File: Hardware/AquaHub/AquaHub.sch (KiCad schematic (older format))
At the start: 73 parts, among them J10 PinHeader6, J13 PinHeader2, J14 PinHeader3, Q2 2SC1815, SW1 SW_Push, SW2 SW_Push, SW3 SW_Push, SW4 SW_Push, SW5 SW_Push, SW6 SW_Push, U1 ESP32-WROOM, U3 1A 3.3V, U4 Low-Side Driver, U5 1A 5V, U6 TCA9534, U7 DS1307+, U8 TPIC2810D, Y1 32.768KHz

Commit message: Commit latest hardware updates and initial firmware
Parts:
- BT1: footprint AquaFootprints:Multicomp-BC-2001 -> Battery:BatteryHolder_Multicomp_BC-2001_1x2032; Mouser (none) -> 534-1058; manf# (none) -> x
- C3: Mouser (none) -> TAJB106K006SNJ; manf# TAJB106K006SNJ -> (none)
- C4: Farnell (none) -> CA06848; Mouser (none) -> TAJD107K006SNJ; manf# TAJD107K006SNJ -> (none)
- C5, C6: Farnell (none) -> CA07886; Mouser (none) -> UWX1H100MCL1GB; manf# UWX1H100MCL1GB -> x
- C7, C8: Mouser (none) -> UWX1H4R7MCL1GB; manf# UWX1H4R7MCL1GB -> x
- C9: Farnell (none) -> CA07658
- LS1: Mouser (none) -> PS1240P02BT; manf# PS1240P02BT -> (none)
- Q2: Farnell (none) -> SC06581
- R10, R11, R12, R13, R14, R15, R16: Farnell (none) -> RE07105; Mouser (none) -> GWCR0603-4K7FT5; manf# GWCR0603-4K7FT5 -> (none)
- R3, R7: Mouser (none) -> GWCR0603-10KFT5; manf# GWCR0603-10KFT5 -> (none)
- R4, R5, R6: manf# GWCR0603-4K7FT5 -> (none)
- R8, R9: Farnell (none) -> RE07090; Mouser (none) -> GWCR0603-4K7FT5; manf# GWCR0603-4K7FT5 -> (none)
- U1: Mouser (none) -> ESP32-WROOM-32D; manf# ESP32-WROOM-32D -> x
- U3: Mouser (none) -> NCP1117DT33G; manf# NCP1117DT33G -> x
- U4: Mouser (none) -> TPL7407LADR; manf# TPL7407LADR -> x
- U5: Mouser (none) -> NCP1117DT50G; manf# NCP1117DT50G -> x
- U6: Mouser (none) -> TCA9534DWR; manf# TCA9534DWR -> x
- U7: manf# (none) -> x
- U8: RS (none) -> 660-7981
- Y1: Mouser (none) -> 815-AB26T-32.768KHZ; manf# (none) -> z

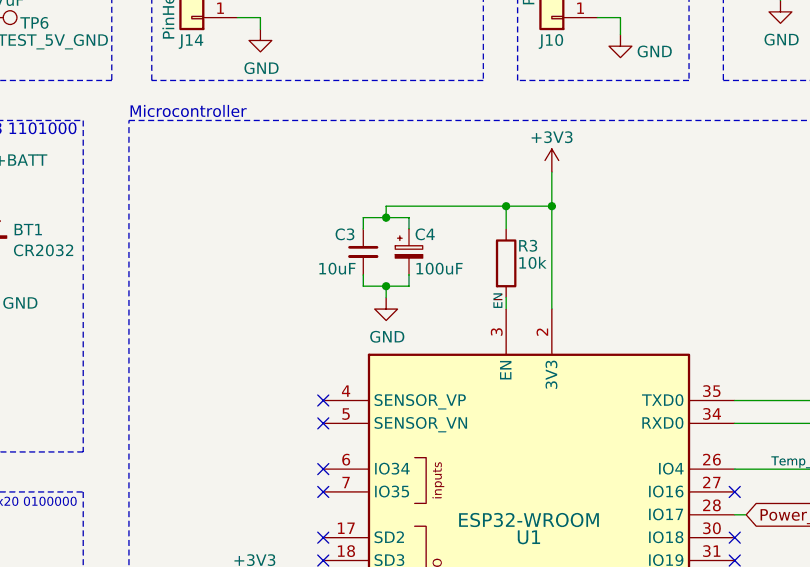
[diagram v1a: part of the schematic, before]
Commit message: Added some more framework
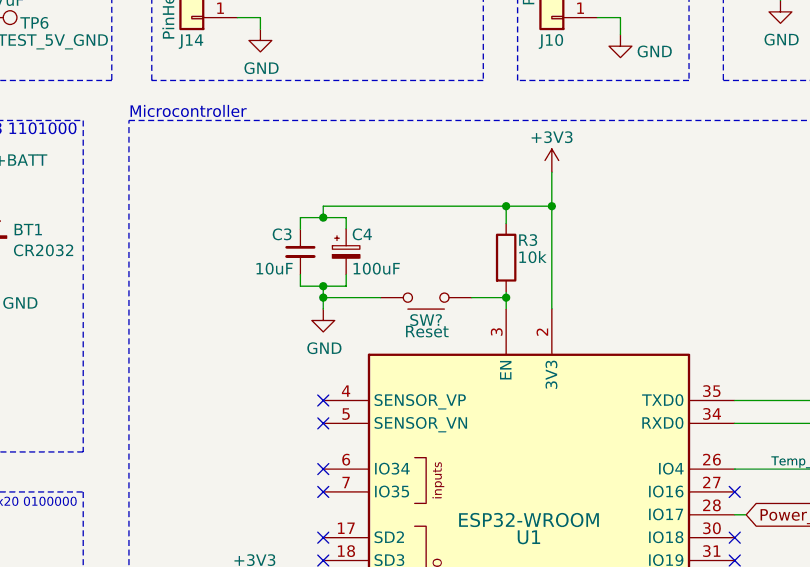
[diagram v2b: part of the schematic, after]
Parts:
- added SW?: Reset, Button_Switch_THT:SW_CK_D6R_SPST_12mm_H14.3mm, symbol AquaHub-rescue:SW_CK_D6R_SPST-Switch
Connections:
- net EN: no longer R3.2, U1.3 (EN)
- net GND: now also SW?.2 (B), SW?.4 (B)
- new net: R3.2, SW?.1 (A), SW?.3 (A), U1.3 (EN)
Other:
- moved on the sheet: C3, C4, R3
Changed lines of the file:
@@
 L AquaHub-rescue:C_Small-Device C3
 U 1 1 5BB06BF9
-P 5525 3250
-F 0 "C3" H 5400 3325 50  0000 L CNN
-F 1 "10uF" H 5325 3175 50  0000 L CNN
-F 2 "Capacitor_SMD:C_0805_2012Metric_Pad1.15x1.40mm_HandSolder" H 5563 3100 50  0001 C CNN
-F 3 "~" H 5525 3250 50  0001 C CNN
-F 4 "Mouser" H 3975 2100 50  0001 C CNN "Vendor"
-F 5 "TAJB106K006SNJ" H 0   0   50  0001 C CNN "Mouser"
-	1    5525 3250
+P 5250 3250
+F 0 "C3" H 5125 3325 50  0000 L CNN
+F 1 "10uF" H 5050 3175 50  0000 L CNN
+F 2 "Capacitor_SMD:C_0805_2012Metric_Pad1.15x1.40mm_HandSolder" H 5288 3100 50  0001 C CNN
+F 3 "~" H 5250 3250 50  0001 C CNN
+F 4 "Mouser" H 3700 2100 50  0001 C CNN "Vendor"
+F 5 "TAJB106K006SNJ" H -275 0   50  0001 C CNN "Mouser"
+	1    5250 3250
 	1    0    0    -1
 $EndComp
@@
 L AquaHub-rescue:CP_Small-Device C4
 U 1 1 5BB06BFF
-P 5725 3250
-F 0 "C4" H 5750 3325 50  0000 L CNN
-F 1 "100uF" H 5750 3175 50  0000 L CNN
-F 2 "Capacitor_Tantalum_SMD:CP_EIA-7343-31_Kemet-D_Pad2.25x2.55mm_HandSolder" H 5763 3100 50  0001 C CNN
-F 3 "~" H 5725 3250 50  0001 C CNN
-F 4 "Mouser" H 3975 2100 50  0001 C CNN "Vendor"
-F 5 "CA06848" H 0   0   50  0001 C CNN "Farnell"
-F 6 "TAJD107K006SNJ" H 0   0   50  0001 C CNN "Mouser"
-	1    5725 3250
-	1    0    0    -1
-$EndComp
-Wire Wire Line
-	5525 3350 5525 3400
-Wire Wire Line
-	5525 3400 5625 3400
-Wire Wire Line
-	5725 3400 5725 3350
-Wire Wire Line
-	5625 3400 5625 3450
-Connection ~ 5625 3400
-Wire Wire Line
-	5625 3400 5725 3400
-Wire Wire Line
-	5525 3150 5525 3100
-Wire Wire Line
-	5525 3100 5625 3100
-Wire Wire Line
-	5725 3100 5725 3150
-Wire Wire Line
-	5625 3100 5625 3050
-Connection ~ 5625 3100
-Wire Wire Line
-	5625 3100 5725 3100
+P 5450 3250
+F 0 "C4" H 5475 3325 50  0000 L CNN
+F 1 "100uF" H 5475 3175 50  0000 L CNN
+F 2 "Capacitor_Tantalum_SMD:CP_EIA-7343-31_Kemet-D_Pad2.25x2.55mm_HandSolder" H 5488 3100 50  0001 C CNN
+F 3 "~" H 5450 3250 50  0001 C CNN
+F 4 "Mouser" H 3700 2100 50  0001 C CNN "Vendor"
+F 5 "CA06848" H -275 0   50  0001 C CNN "Farnell"
+F 6 "TAJD107K006SNJ" H -275 0   50  0001 C CNN "Mouser"
+	1    5450 3250
+	1    0    0    -1
+$EndComp
+Wire Wire Line
+	5250 3350 5250 3400
+Wire Wire Line
+	5250 3400 5350 3400
+Wire Wire Line
+	5450 3400 5450 3350
+Connection ~ 5350 3400
+Wire Wire Line
+	5350 3400 5450 3400
+Wire Wire Line
+	5250 3150 5250 3100
+Wire Wire Line
+	5250 3100 5350 3100
+Wire Wire Line
+	5450 3100 5450 3150
+Wire Wire Line
+	5350 3100 5350 3050
+Connection ~ 5350 3100
+Wire Wire Line
+	5350 3100 5450 3100
 $Comp
 L AquaHub-rescue:GND-power #PWR0106
 U 1 1 5BB06C11
-P 5625 3450
-F 0 "#PWR0106" H 5625 3200 50  0001 C CNN
-F 1 "GND" H 5630 3277 50  0000 C CNN
-F 2 "" H 5625 3450 50  0001 C CNN
-F 3 "" H 5625 3450 50  0001 C CNN
-	1    5625 3450
-	1    0    0    -1
-$EndComp
-Wire Wire Line
-	5625 3050 6150 3050
+P 5350 3500
+F 0 "#PWR0106" H 5350 3250 50  0001 C CNN
+F 1 "GND" H 5355 3327 50  0000 C CNN
+F 2 "" H 5350 3500 50  0001 C CNN
+F 3 "" H 5350 3500 50  0001 C CNN
+	1    5350 3500
+	1    0    0    -1
+$EndComp
 $Comp
 L AquaHub-rescue:Conn_01x02-Connector_Generic J13
@@
 L AquaHub-rescue:R-Device R3
 U 1 1 5BA87CFB
-P 6150 3300
-F 0 "R3" H 6200 3375 50  0000 L CNN
-F 1 "10k" H 6200 3300 50  0000 L CNN
-F 2 "Resistor_SMD:R_0603_1608Metric_Pad1.05x0.95mm_HandSolder" V 6080 3300 50  0001 C CNN
-F 3 "~" H 6150 3300 50  0001 C CNN
-F 4 "Mouser" H 3975 2100 50  0001 C CNN "Vendor"
-F 5 "GWCR0603-10KFT5" H 0   0   50  0001 C CNN "Mouser"
-	1    6150 3300
-	1    0    0    -1
-$EndComp
-Text Label 6150 3500 1    39   ~ 0
-EN
+P 6150 3275
+F 0 "R3" H 6200 3350 50  0000 L CNN
+F 1 "10k" H 6200 3275 50  0000 L CNN
+F 2 "Resistor_SMD:R_0603_1608Metric_Pad1.05x0.95mm_HandSolder" V 6080 3275 50  0001 C CNN
+F 3 "~" H 6150 3275 50  0001 C CNN
+F 4 "Mouser" H 3975 2075 50  0001 C CNN "Vendor"
+F 5 "GWCR0603-10KFT5" H 0   -25 50  0001 C CNN "Mouser"
+	1    6150 3275
+	1    0    0    -1
+$EndComp
 $Comp
 L AquaHub-rescue:R-Device R7
@@
 	7425 4700 7150 4700
 Wire Wire Line
-	6150 3150 6150 3050
+	6150 3125 6150 3050
 Wire Wire Line
 	6150 3050 6350 3050
@@
 	6350 3050 6350 2900
 Wire Wire Line
-	6150 3450 6150 3500
-Connection ~ 6150 3050
+	6150 3425 6150 3450
 Wire Wire Line
 	4875 5300 4900 5300
@@
 NoConn ~ 5350 4000
 NoConn ~ 5350 3900
+$Comp
+L AquaHub-rescue:SW_CK_D6R_SPST-Switch SW?
+U 1 1 5BD9B1CF
+P 5800 3450
+AR Path="/5B8F2634/5BD9B1CF" Ref="SW?"  Part="1"
+AR Path="/5BD9B1CF" Ref="SW?"  Part="1"
+F 0 "SW?" H 5800 3550 50  0000 C CNN
+F 1 "Reset" H 5700 3600 50  0000 L CNN
+F 2 "Button_Switch_THT:SW_CK_D6R_SPST_12mm_H14.3mm" H 5800 3650 50  0001 C CNN
+F 3 "" H 5800 3650 50  0001 C CNN
+F 4 "Mouser" H -1175 -875 50  0001 C CNN "Vendor"
+	1    5800 3450
+	-1   0    0    1
+$EndComp
+Wire Wire Line
+	5350 3050 6150 3050
+Wire Wire Line
+	6150 3450 6000 3450
+Connection ~ 6150 3450
+Wire Wire Line
+	6150 3450 6150 3500
+Wire Wire Line
+	5350 3400 5350 3450
+Wire Wire Line
+	5600 3450 5350 3450
+Connection ~ 5350 3450
+Wire Wire Line
+	5350 3450 5350 3500
+Connection ~ 6150 3050
 $EndSCHEMATC
